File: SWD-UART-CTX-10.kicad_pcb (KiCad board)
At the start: 2 copper layers, 23.6 x 26.4 mm, 13 parts, among them J1 61300611121, J2 3020-10-0100-00, J3 SFH11-PBPC-D10-RA-BK, J4 61300211121

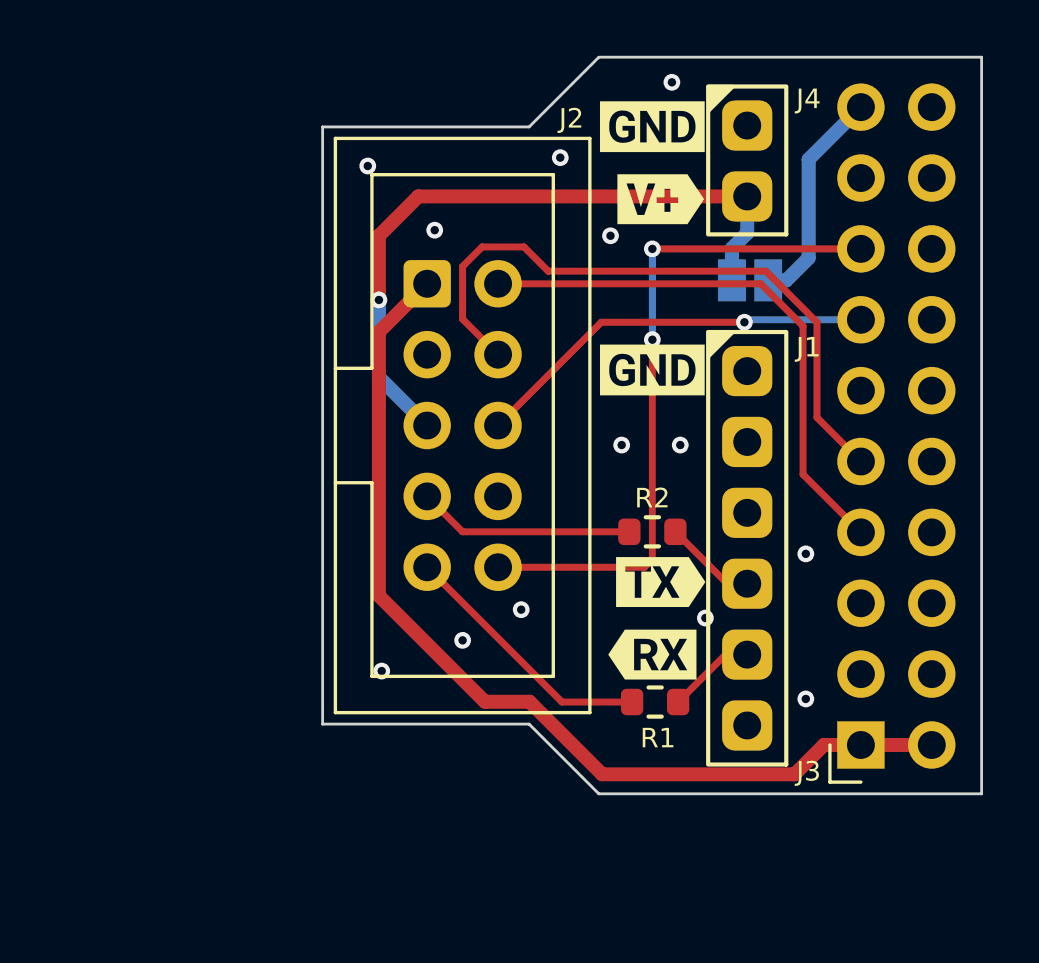
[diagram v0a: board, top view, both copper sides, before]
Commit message: Update for J-Link options
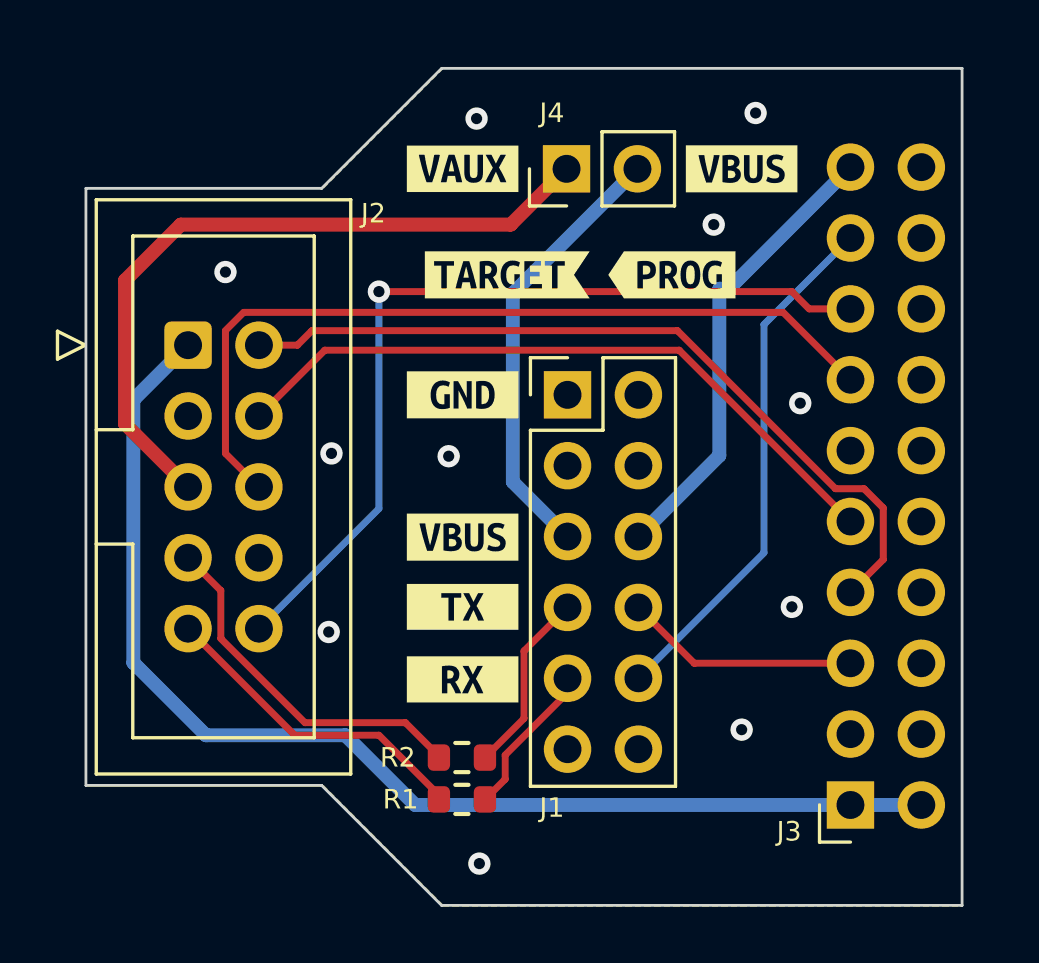
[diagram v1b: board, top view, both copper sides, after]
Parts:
- removed JP1: SolderJumper_2_Open, Jumper:SolderJumper-2_P1.3mm_Open_Pad1.0x1.5mm
- removed kibuzzard-637893A0: G***, kibuzzard-637893A0
- removed kibuzzard-637893BE: G***, kibuzzard-637893BE
- removed kibuzzard-637893D0 (x2): G***, kibuzzard-637893D0
- removed kibuzzard-637893E3: G***, kibuzzard-637893E3
- added kibuzzard-653C8A9D: G***, kibuzzard-653C8A9D, F.Cu at (131.4, 92.1)
- added kibuzzard-653C8AA8: G***, kibuzzard-653C8AA8, F.Cu at (131.4, 97.2)
- added kibuzzard-653C8AB2: G***, kibuzzard-653C8AB2, F.Cu at (131.4, 99.7)
- added kibuzzard-653C8ABC: G***, kibuzzard-653C8ABC, F.Cu at (131.4, 102.3)
- added kibuzzard-653C8B0E: G***, kibuzzard-653C8B0E, F.Cu at (131.4, 84.0)
- added kibuzzard-653C8B17: G***, kibuzzard-653C8B17, F.Cu at (141.4, 84.0)
- added kibuzzard-653C8B44: G***, kibuzzard-653C8B44, F.Cu at (138.9, 87.8)
- added kibuzzard-653C8BB4: G***, kibuzzard-653C8BB4, F.Cu at (133.0, 87.8)
- J1: value 61300611121 -> 61301221121; footprint J_Connector:Pins-2.54-1x6 -> Connector_PinHeader_2.54mm:PinHeader_2x06_P2.54mm_Vertical
- J4: footprint J_Connector:Pins-2.54-1x2 -> Connector_PinHeader_2.54mm:PinHeader_1x02_P2.54mm_Vertical
- moved R2 10.6 mm to (131.4, 105.1)
- moved J2 8.85 mm to (121.6, 90.3)
- moved R1 7.75 mm to (131.4, 106.6)
- moved ~ 7.12 mm to (130.2, 103.2)
- moved J4 6.66 mm to (135.1, 84.0), turned to 90 degrees
- moved J1 6.50 mm to (135.2, 92.1)
- moved J3 2.18 mm to (145.3, 106.8)
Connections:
- J1 pad 2: unconnected-(J1-Pad2) -> GND
- J1 pad 4: Net-(J1-Pad4) -> unconnected-(J1-Pin_4-Pad4)
- J1 pad 5: Net-(J1-Pad5) -> /VBUS
- J1 pad 6: unconnected-(J1-Pad6) -> /VBUS_PROG
- J3 pad 17: unconnected-(J3-Pad17) -> /RXD_PROG
- J3 pad 19: Net-(J3-Pad19) -> /VBUS_PROG
- J3 pad 5: unconnected-(J3-Pad5) -> /TXD_PROG
- J4 pad 1: GND -> /VAUX
- J4 pad 2: /VAUX -> /VBUS
- R1 pad 2: Net-(J1-Pad5) -> Net-(J1-Pin_9)
- R2 pad 2: Net-(J1-Pad4) -> Net-(J1-Pin_7)
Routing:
- net /RXD_PROG: track 0.00 -> 18.9 mm
- net /VBUS_PROG: track 0.00 -> 16.6 mm
- net /VBUS: track 0.00 -> 15.8 mm
- net /SWO: track 14.6 -> 29.8 mm, vias 1 -> 0
- net /SWDIO: track 19.8 -> 28.7 mm
- net /TXD_PROG: track 0.00 -> 8.43 mm
- net Net-(J3-Pad19): track 7.97 -> 0.00 mm
- net /TARGET_VCC: track 34.8 -> 42.5 mm
- net /RESET: track 24.3 -> 31.0 mm, vias 2 -> 1
- net Net-(J1-Pin_7): track 0.00 -> 6.61 mm
- net Net-(J1-Pin_9): track 0.00 -> 5.57 mm
- net /TXD: track 7.77 -> 13.0 mm
- net Net-(J1-Pad4): track 3.35 -> 0.00 mm
- net Net-(J1-Pad5): track 3.18 -> 0.00 mm
- net /RXD: track 9.35 -> 11.6 mm
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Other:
- board size 23.6 x 26.4 mm -> 31.4 x 30 mm
- board text added: "SWD-UART-CTX-10 v2.0 Oct 23"
- board text removed: "SWD-UART-CTX-10 V1.1 Nov 22"
- board text removed: "VAUX-VBUS"
